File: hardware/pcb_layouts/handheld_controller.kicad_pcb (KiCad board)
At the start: 2 copper layers, 6 parts, among them SW1 SW_SP3T, SW2 SW_SP3T, SW3 SW_SP3T, SW4 SW_SP3T, SW6 SW_SPDT, U1 ESP32-S3-DEVKITC-1-N8R8

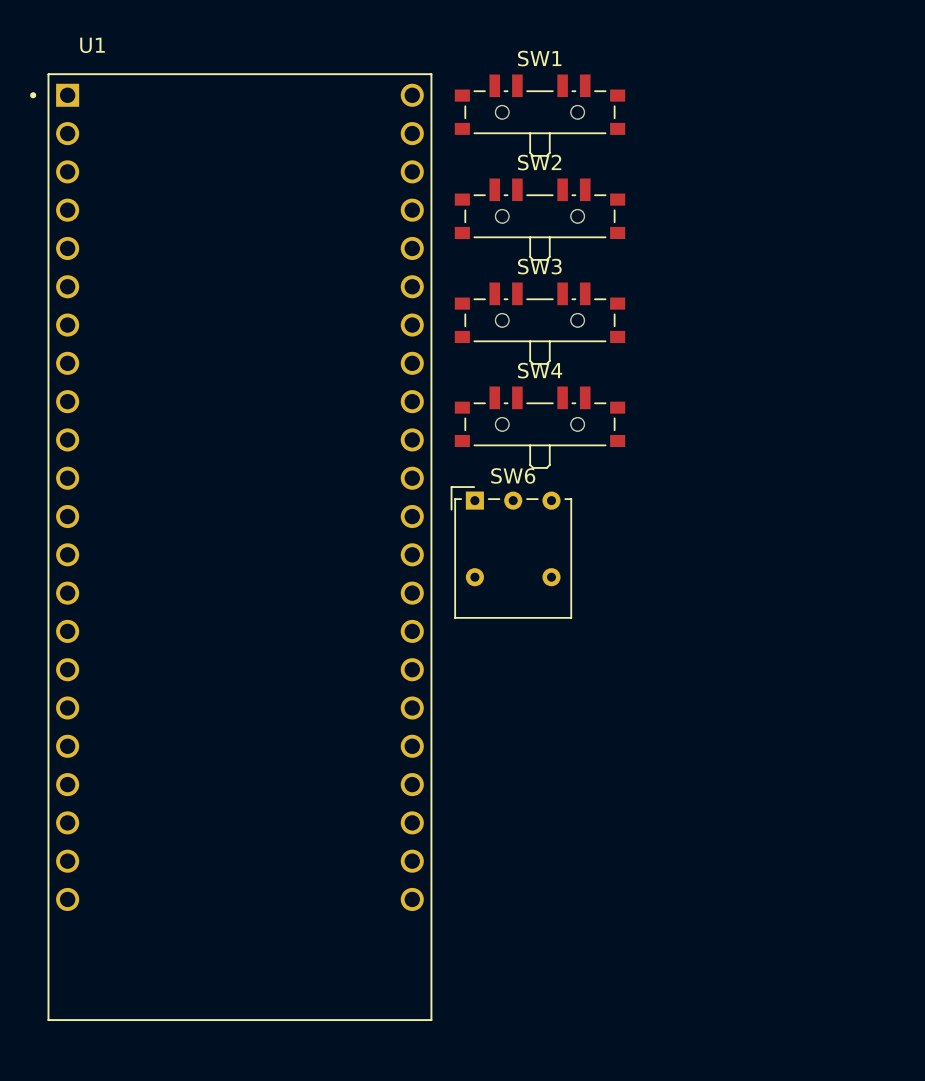
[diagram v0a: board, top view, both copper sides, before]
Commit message: acceptably final PCB (passes DRC)
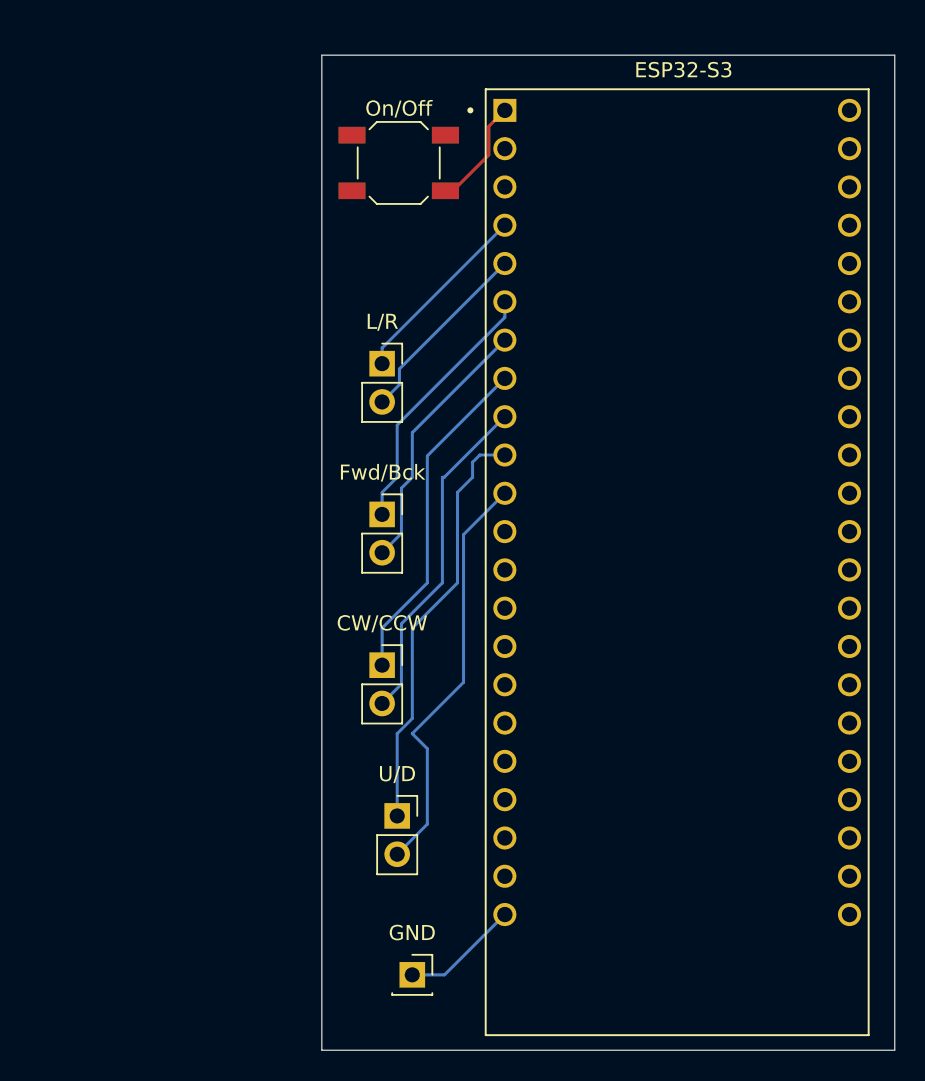
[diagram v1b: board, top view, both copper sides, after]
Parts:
- removed SW1, SW2, SW3, SW4: SW_SP3T, Button_Switch_SMD:SW_SP3T_PCM13
- removed SW6: SW_SPDT, Button_Switch_THT:SW_Lever_1P2T_NKK_GW12LxH
- removed U1: ESP32-S3-DEVKITC-1-N8R8, ESP32-S3-DEVKITC-1-N8R8:ESP32-S3-DEVKITC-1-N8R8
- added CW/CCW: Conn_01x02_Pin, Connector_PinSocket_2.54mm:PinSocket_1x02_P2.54mm_Vertical, F.Cu at (149.0, 107.5)
- added ESP32-S3: ESP32-S3-DEVKITC-1-N8R8, ESP32-S3-DEVKITC-1-N8R8:ESP32-S3-DEVKITC-1-N8R8, F.Cu at (168.6, 100.6)
- added Fwd/Bck: Conn_01x02_Pin, Connector_PinSocket_2.54mm:PinSocket_1x02_P2.54mm_Vertical, F.Cu at (149.0, 97.5)
- added GND: Conn_01x01_Pin, Connector_PinSocket_2.54mm:PinSocket_1x01_P2.54mm_Vertical, F.Cu at (151.0, 128.0)
- added L/R : Conn_01x02_Pin, Connector_PinSocket_2.54mm:PinSocket_1x02_P2.54mm_Vertical, F.Cu at (149.0, 87.5)
- added On/Off: SW_DIP_x01, Button_Switch_SMD:SW_SPST_SKQG_WithStem, F.Cu at (150.1, 74.2)
- added U/D: Conn_01x02_Pin, Connector_PinSocket_2.54mm:PinSocket_1x02_P2.54mm_Vertical, F.Cu at (150.0, 117.5)
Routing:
- net Net-(J4-Pin_1): track 0.00 -> 27.9 mm
- net Net-(J4-Pin_2): track 0.00 -> 27.7 mm
- net Net-(J3-Pin_2): track 0.00 -> 22.5 mm
- net Net-(J3-Pin_1): track 0.00 -> 22.4 mm
- net Net-(J2-Pin_2): track 0.00 -> 17.5 mm
- net Net-(J2-Pin_1): track 0.00 -> 17.5 mm
- net Net-(J1-Pin_2): track 0.00 -> 12.6 mm
- net Net-(J1-Pin_1): track 0.00 -> 12.6 mm
- net GND: track 0.00 -> 7.80 mm
- net Net-(U1-3V3): track 0.00 -> 7.26 mm
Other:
- board outline added: 38 x 66 mm
